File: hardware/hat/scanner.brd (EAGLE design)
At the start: 65 x 56 mm, 30 parts, among them J1 PJ-102AH, U1 CAT24C32WI-GT3, U2 TPS61165DBV

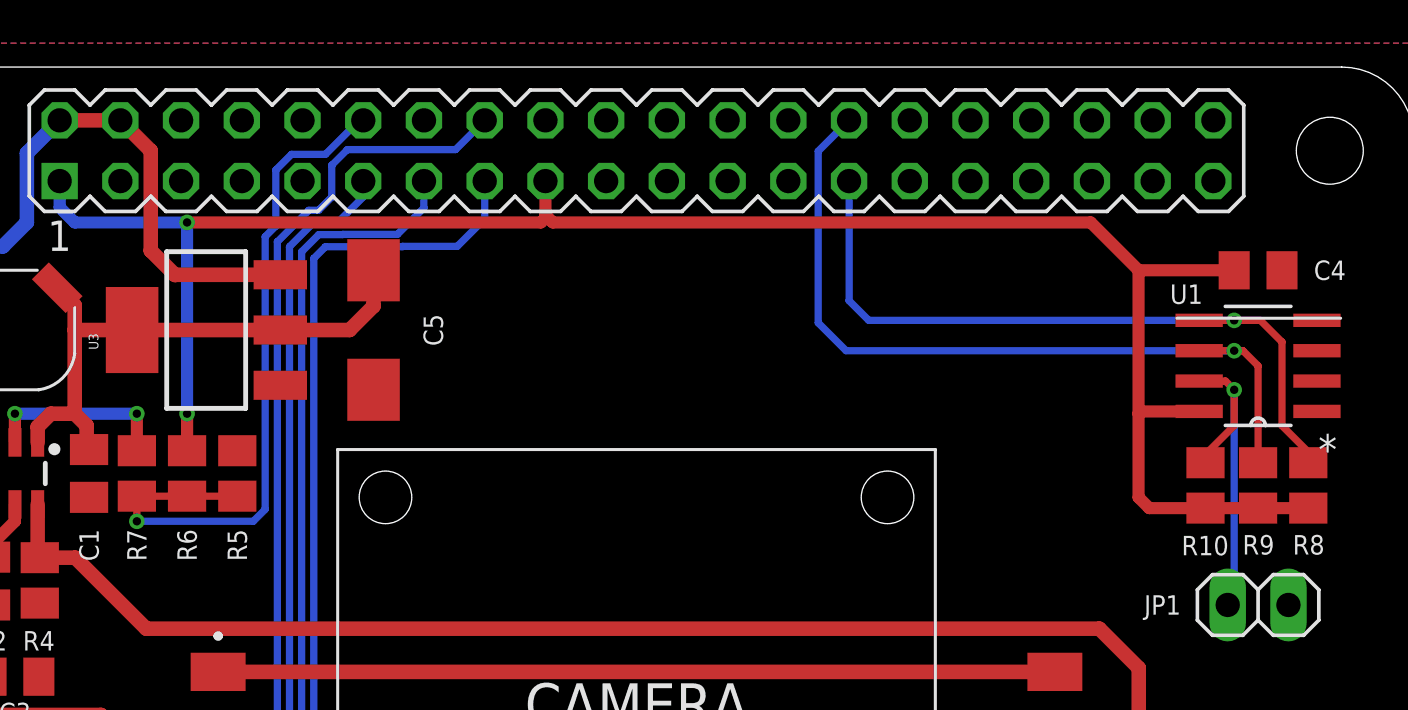
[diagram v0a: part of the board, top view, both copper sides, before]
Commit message: tweak layout
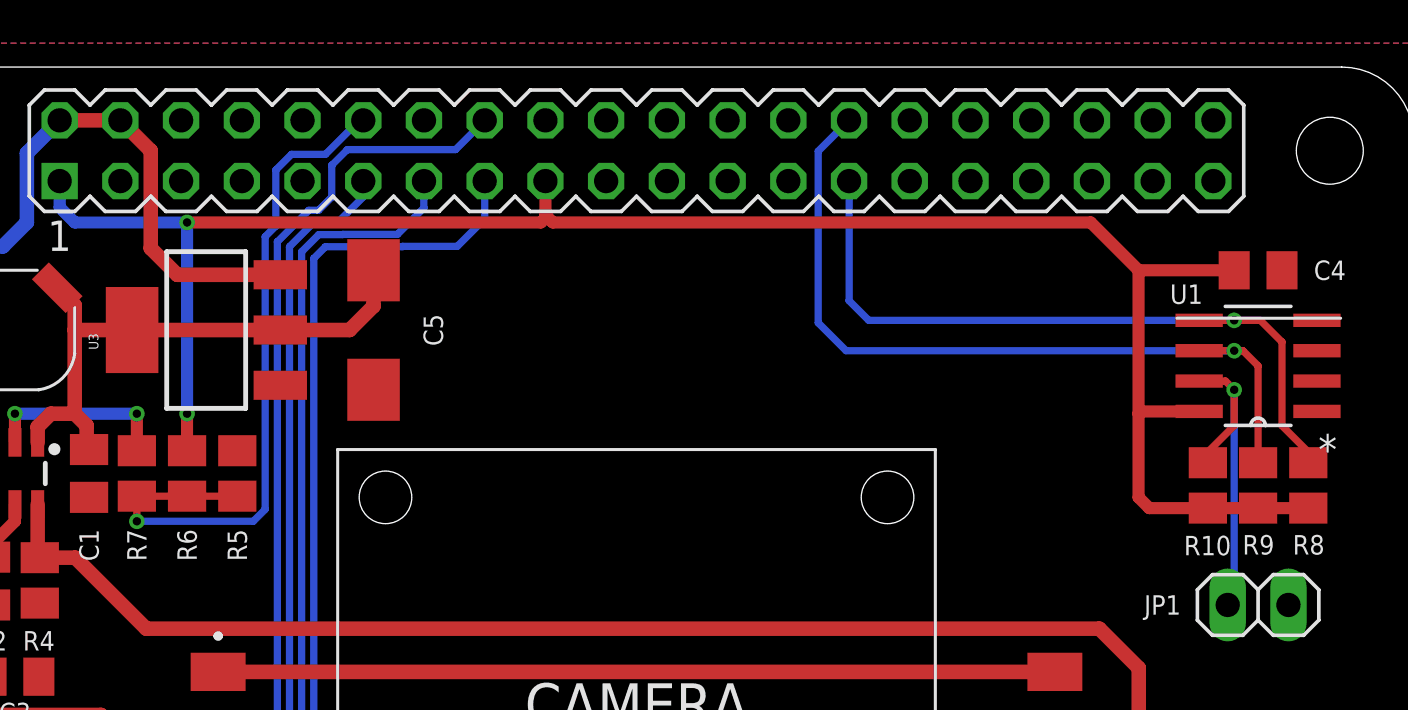
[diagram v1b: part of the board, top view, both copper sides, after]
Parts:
- moved R10 0.10 mm to (23.9, -14.0)
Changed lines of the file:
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@@
 <attribute name="VALUE" x="29.4544" y="-3.285" size="2.0828" layer="27" ratio="10" rot="SR180"/>
 </element>
-<element name="R10" library="resistor" package="M0805" value="3k9" x="23.8" y="-14" smashed="yes" rot="R90">
-<attribute name="NAME" x="23.784" y="-16.516" size="0.8128" layer="25" font="fixed" rot="R180" align="center"/>
-<attribute name="TOLERANCE" value="5%" x="26.0225" y="-35.59" size="1.778" layer="27" rot="R90" display="off"/>
-<attribute name="VALUE" x="26.086" y="-15.016" size="1.27" layer="27" rot="R90"/>
+<element name="R10" library="resistor" package="M0805" value="3k9" x="23.9" y="-14" smashed="yes" rot="R90">
+<attribute name="NAME" x="23.884" y="-16.516" size="0.8128" layer="25" font="fixed" rot="R180" align="center"/>
+<attribute name="TOLERANCE" value="5%" x="26.1225" y="-35.59" size="1.778" layer="27" rot="R90" display="off"/>
+<attribute name="VALUE" x="26.186" y="-15.016" size="1.27" layer="27" rot="R90"/>
 </element>
 <element name="JP1" library="pinhead" library_urn="urn:adsk.eagle:library:325" package="1X02" package3d_urn="urn:adsk.eagle:package:22435/2" value="" x="26" y="-19" smashed="yes">
@@
 <contactref element="R10" pad="1"/>
 <wire x1="28.1" y1="-14.95" x2="26" y2="-14.95" width="0.508" layer="1"/>
-<wire x1="26" y1="-14.95" x2="23.8" y2="-14.95" width="0.508" layer="1"/>
-<wire x1="23.8" y1="-14.95" x2="21.45" y2="-14.95" width="0.508" layer="1"/>
+<wire x1="26" y1="-14.95" x2="23.9" y2="-14.95" width="0.508" layer="1"/>
+<wire x1="23.9" y1="-14.95" x2="21.45" y2="-14.95" width="0.508" layer="1"/>
 <wire x1="21.45" y1="-14.95" x2="21" y2="-14.5" width="0.508" layer="1"/>
 <wire x1="21" y1="-5" x2="21" y2="-11" width="0.508" layer="1"/>
@@
 <wire x1="-21.59" y1="1.27" x2="-24.13" y2="1.27" width="0.6096" layer="1"/>
 <wire x1="-20.32" y1="0" x2="-21.59" y2="1.27" width="0.6096" layer="1"/>
-<wire x1="-19.3" y1="-5.2" x2="-20.32" y2="-4.18" width="0.6096" layer="1"/>
-<wire x1="-20.32" y1="-4.18" x2="-20.32" y2="0" width="0.6096" layer="1"/>
+<wire x1="-19.2114" y1="-5.1886" x2="-20.32" y2="-4.08" width="0.6096" layer="1"/>
+<wire x1="-20.32" y1="-4.08" x2="-20.32" y2="0" width="0.6096" layer="1"/>
 <contactref element="U3" pad="3"/>
-<wire x1="-14.9012" y1="-5.1886" x2="-19.2886" y2="-5.1886" width="0.6096" layer="1"/>
-<wire x1="-19.2886" y1="-5.1886" x2="-19.3" y2="-5.2" width="0.6096" layer="1"/>
+<wire x1="-14.9012" y1="-5.1886" x2="-19.2114" y2="-5.1886" width="0.6096" layer="1"/>
 <contactref element="C6" pad="+"/>
 <contactref element="J1" pad="1"/>
@@
 <contactref element="JP1" pad="1"/>
 <contactref element="R10" pad="2"/>
-<wire x1="23.8" y1="-13.05" x2="23.8" y2="-12.7" width="0.3048" layer="1"/>
-<wire x1="25" y1="-11.5" x2="23.8" y2="-12.7" width="0.3048" layer="1"/>
+<wire x1="23.9" y1="-13.05" x2="23.9" y2="-12.6" width="0.3048" layer="1"/>
+<wire x1="25" y1="-11.5" x2="23.9" y2="-12.6" width="0.3048" layer="1"/>
 <wire x1="23.5362" y1="-9.635" x2="24.635" y2="-9.635" width="0.3048" layer="1"/>
 <wire x1="24.635" y1="-9.635" x2="25" y2="-10" width="0.3048" layer="1"/>
